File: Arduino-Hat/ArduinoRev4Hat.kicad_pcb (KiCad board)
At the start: 2 copper layers, 42.8 x 83.5 mm, 12 parts, among them J1 Conn_01x10_Pin, J10 73099-0, J11 73099-0, J2 Conn_01x08_Pin, J3 Conn_01x04_Pin, J4 Conn_01x04_Pin, J5 Conn_01x04_Pin, J6 73099-0, J7 73099-0, J8 73099-0, J9 73099-0

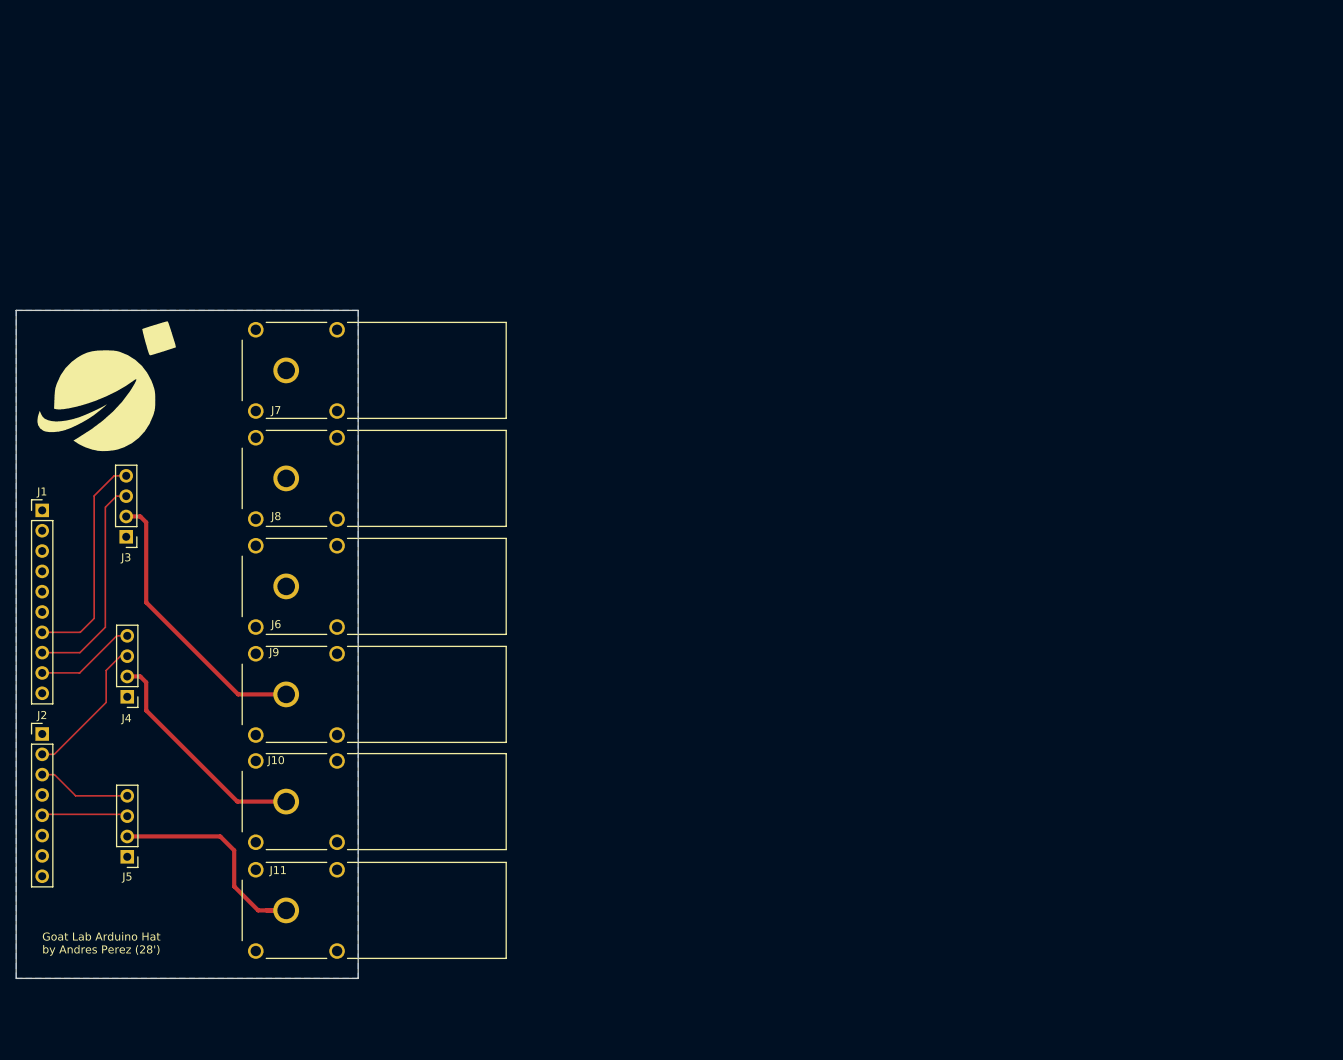
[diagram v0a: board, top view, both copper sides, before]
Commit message: updates pcb for arduino
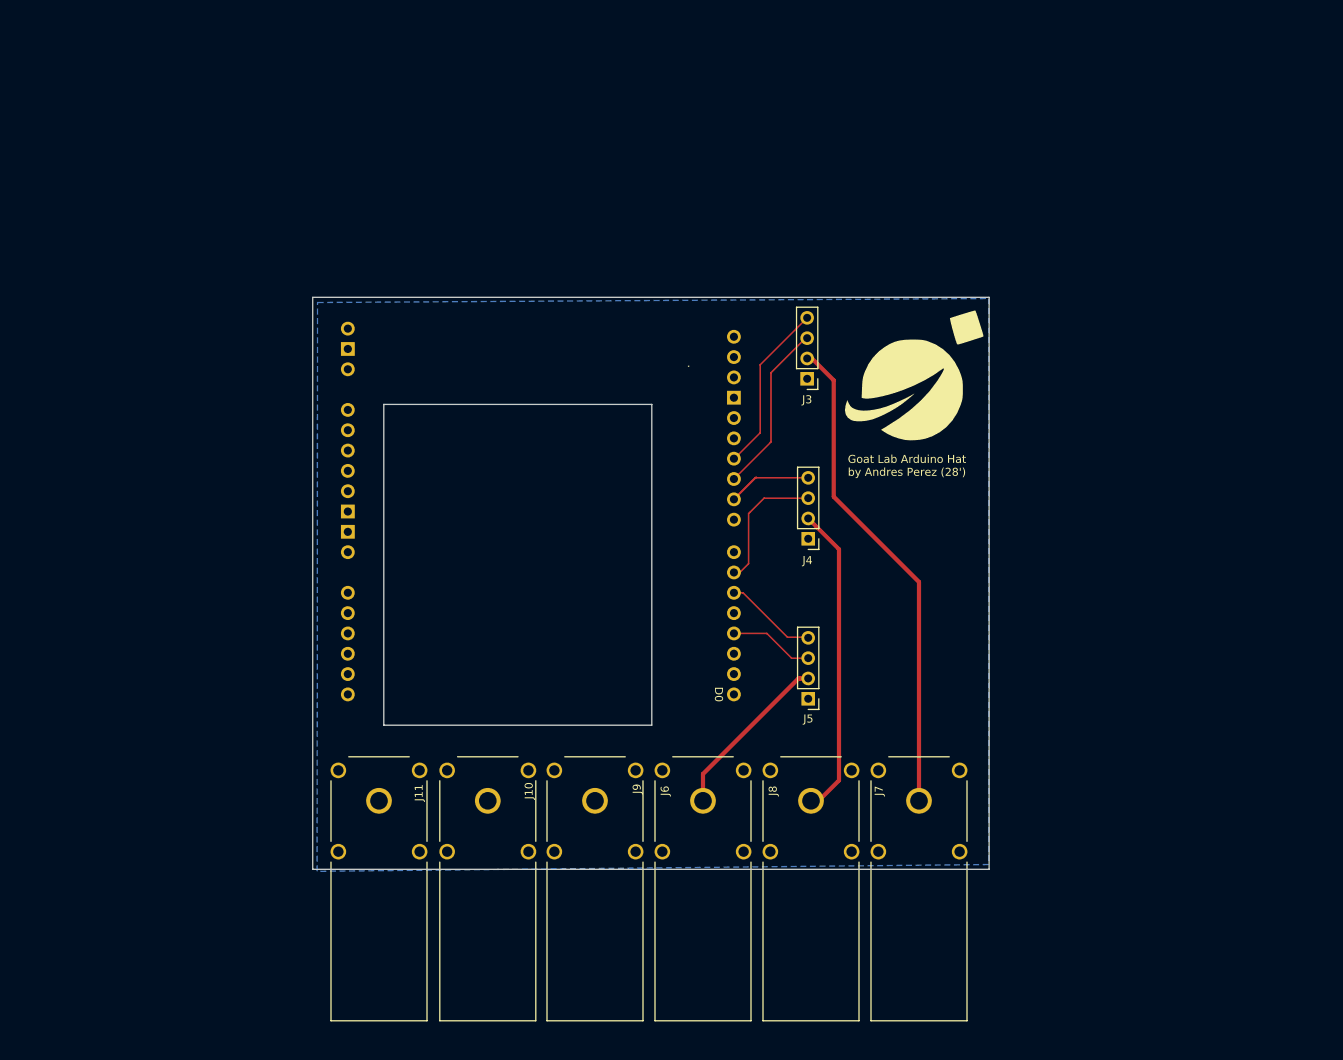
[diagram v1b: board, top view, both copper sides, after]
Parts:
- removed J1: Conn_01x10_Pin, Connector_PinHeader_2.54mm:PinHeader_1x10_P2.54mm_Vertical
- removed J2: Conn_01x08_Pin, Connector_PinHeader_2.54mm:PinHeader_1x08_P2.54mm_Vertical
- added A1: Arduino_Uno_R4_WiFi_Shield, my_custom:Arduino_Uno_R4_WiFi_Shield, F.Cu at (106.2, 40.0)
- moved G*** 101.0 mm to (179.4, 63.6)
- moved J7 95.7 mm to (180.1, 116.8), turned to -90 degrees
- moved J3 87.4 mm to (166.1, 64.0)
- moved J4 87.4 mm to (166.2, 84.0)
- moved J5 87.4 mm to (166.2, 104.0)
- moved J8 77.0 mm to (166.6, 116.8), turned to -90 degrees
- moved J6 58.6 mm to (153.1, 116.8), turned to -90 degrees
- moved J9 40.8 mm to (139.6, 116.8), turned to -90 degrees
- moved J10 25.2 mm to (126.2, 116.8), turned to -90 degrees
- moved J11 18.0 mm to (112.6, 116.8), turned to -90 degrees
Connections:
- J10 pad 1: /VM_Y -> GND
- J11 pad 1: /VM_Z -> GND
- J6 pad 1: GND -> /VM_Z
- J7 pad 1: GND -> /VM_X
- J8 pad 1: GND -> /VM_Y
- J9 pad 1: /VM_X -> GND
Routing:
- net /VM_X: track 35.1 -> 61.4 mm
- net /VM_Y: track 28.4 -> 40.0 mm
- net /IN2_X: track 28.1 -> 21.4 mm
- net /IN1_X: track 27.4 -> 21.5 mm
- net /VM_Z: track 28.8 -> 23.7 mm
- net /IN2_Y: track 12.6 -> 14.3 mm
- net /IN1_Y: track 18.1 -> 16.8 mm
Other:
- board size 42.8 x 83.5 mm -> 84.5 x 71.5 mm

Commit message: newest version
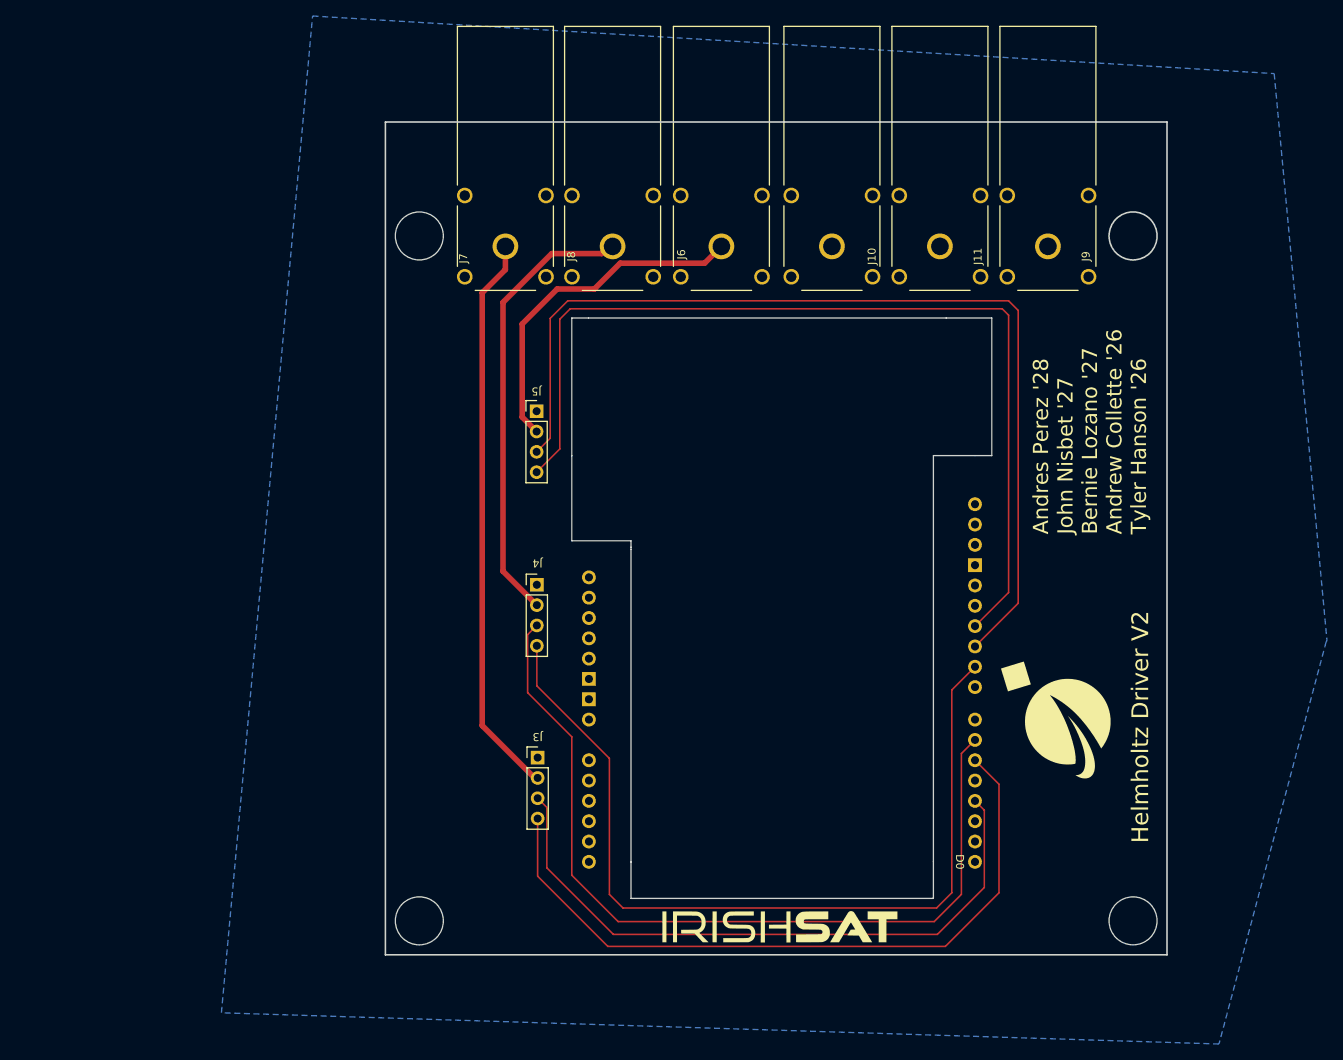
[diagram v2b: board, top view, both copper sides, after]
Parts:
- removed the G*** at (179.4, 63.6)
- added G***: LOGO, LOGO, F.Cu at (197.2, 106.7)
- added G***: LOGO, LOGO, F.Cu at (162.5, 132.6)
- moved J9 81.6 mm to (196.2, 47.5), turned to 90 degrees
- moved J6 81.5 mm to (155.4, 47.5), turned to 90 degrees
- moved J11 71.2 mm to (182.7, 47.5), turned to 90 degrees
- moved J8 71.0 mm to (141.8, 47.5), turned to 90 degrees
- moved J7 70.2 mm to (128.4, 47.5), turned to 90 degrees
- moved J10 70.2 mm to (169.2, 47.5), turned to 90 degrees
- moved J3 58.1 mm to (132.4, 111.4), turned to 0 degrees
- moved J5 49.4 mm to (132.3, 68.1), turned to 0 degrees
- moved A1 36.7 mm to (136.3, 60.9)
- moved J4 34.4 mm to (132.3, 89.8), turned to 0 degrees
- renumbered J7 to J10, J8 to J11, J11 to J6, J9 to J7, J10 to J8, J6 to J9
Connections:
- A1 pad GND1: unconnected-(A1-GND-PadGND1) -> GND
- A1 pad GND2: unconnected-(A1-GND-PadGND2) -> GND
- J10 pad 1: /VM_X -> GND
- J11 pad 1: /VM_Y -> GND
- J3 pad 2: /VM_X -> /VM_Z
- J3 pad 3: /IN1_X -> /IN1_Z
- J3 pad 4: /IN2_X -> /IN2_Z
- J5 pad 2: /VM_Z -> /VM_X
- J5 pad 3: /IN1_Z -> /IN1_X
- J5 pad 4: /IN2_Z -> /IN2_X
- J6 pad 1: GND -> /VM_X
- J7 pad 1: GND -> /VM_Z
- J8 pad 1: GND -> /VM_Y
- J9 pad 1: /VM_Z -> GND
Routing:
- net /IN1_X: track 21.5 -> 121.5 mm
- net /IN2_X: track 21.4 -> 117.9 mm
- net /IN2_Y: track 14.3 -> 108.6 mm
- net /IN1_Y: track 16.8 -> 106.5 mm
- net /IN2_Z: track 11.5 -> 89.1 mm
- net /IN1_Z: track 10.6 -> 81.0 mm
- net /VM_Z: track 23.7 -> 70.7 mm
- net /VM_X: track 61.4 -> 43.1 mm
- net /VM_Y: track 40.0 -> 56.2 mm
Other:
- board size 84.5 x 71.5 mm -> 97.7 x 104.1 mm
- board text added: "Andres Perez '28 John Nisbet '27 Bernie Lozano '27 Andrew Collette '26 Tyler Hanson '26"
- board text added: "Helmholtz Driver V2"
- board text removed: "Goat Lab Arduino Hat by Andres Perez (28')"
